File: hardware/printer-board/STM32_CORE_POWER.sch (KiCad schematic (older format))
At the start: 8 parts, among them U14 AMS1117-3.3

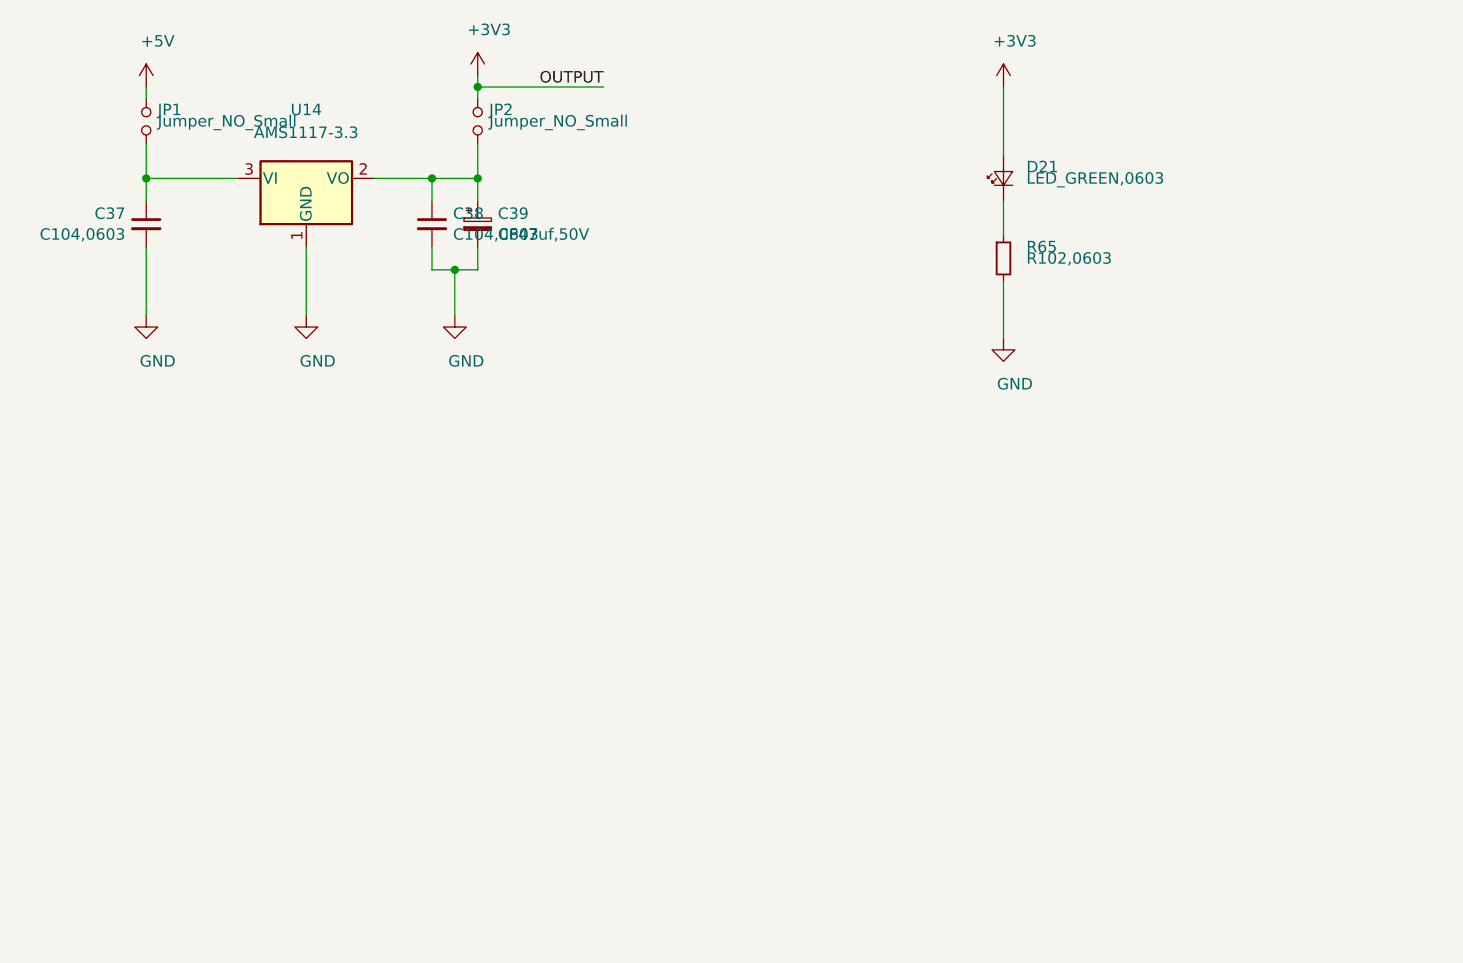
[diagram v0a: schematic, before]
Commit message: update,
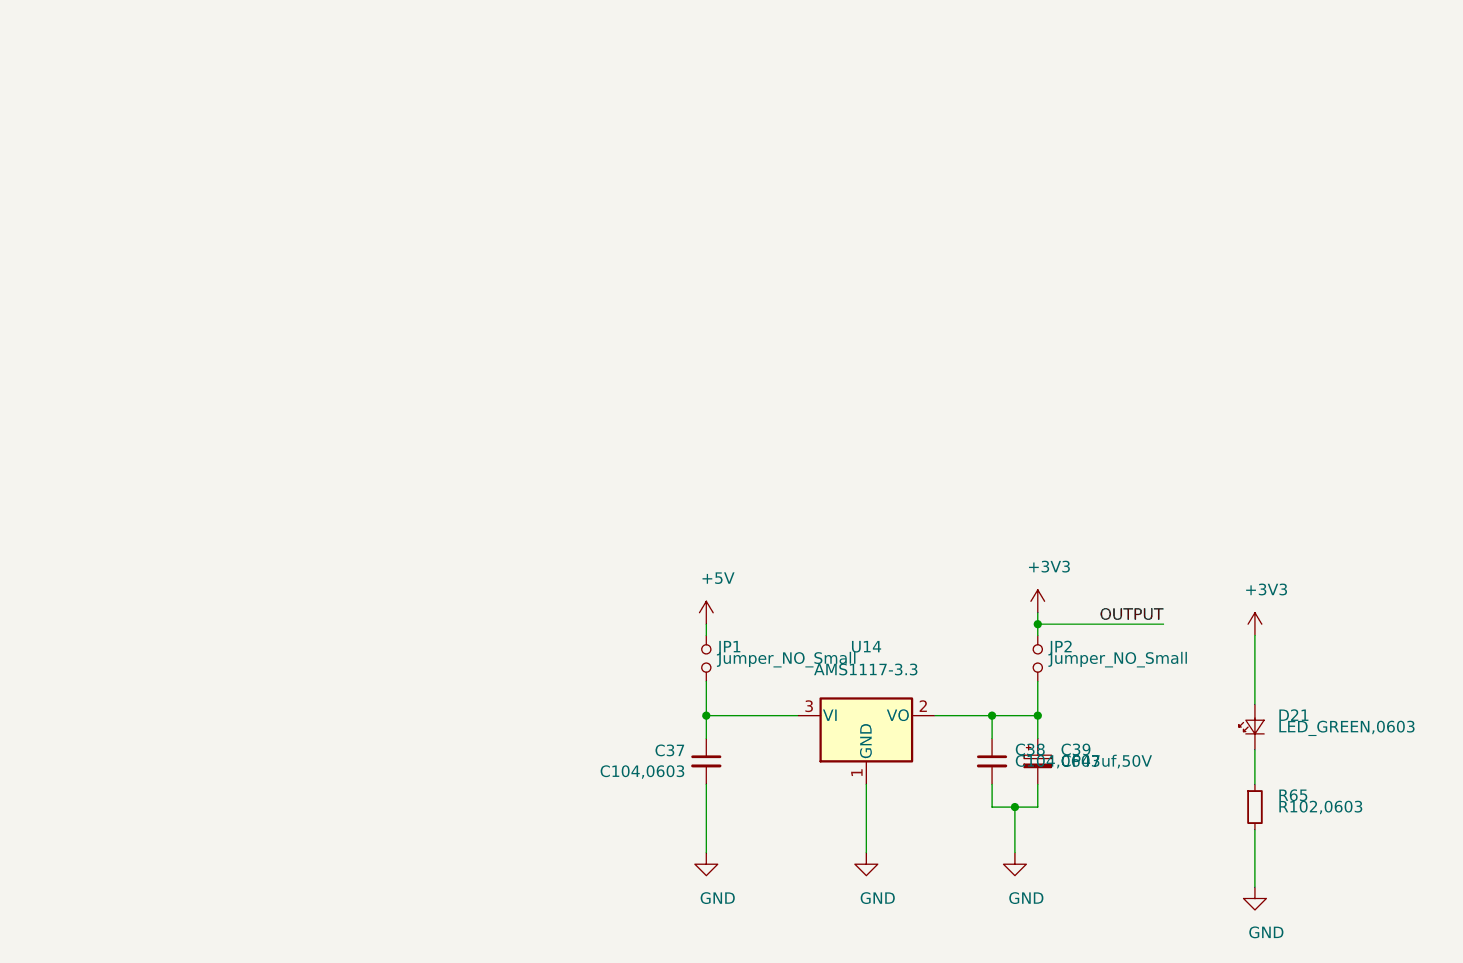
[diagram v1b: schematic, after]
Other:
- moved on the sheet: C37, C38, C39, D21, JP1, JP2, R65, U14
